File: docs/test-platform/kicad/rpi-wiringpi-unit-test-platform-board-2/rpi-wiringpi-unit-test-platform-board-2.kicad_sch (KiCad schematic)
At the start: 22 parts, among them J1 IN_PWR, J2 IN_SIGNAL, J3 IN_CS_SHIFTREG, J4 OUT_SERVO, J5 OUT_SERVO_SIG, SW1 SW_BOARD_CONN_LED, U1 MCP3008, U2 MCP4922, U3 MCP42010, U4 ADS1115, U5 74HC595

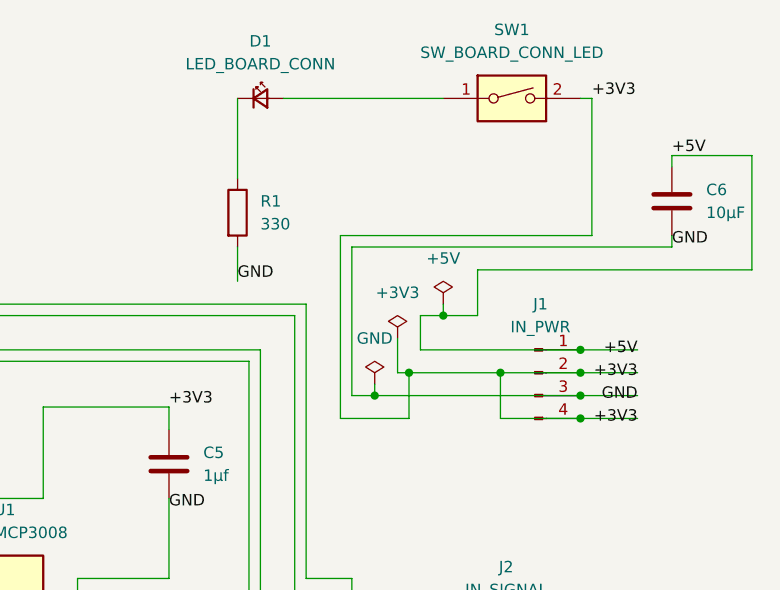
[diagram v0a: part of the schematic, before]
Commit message: Cleanup tracing
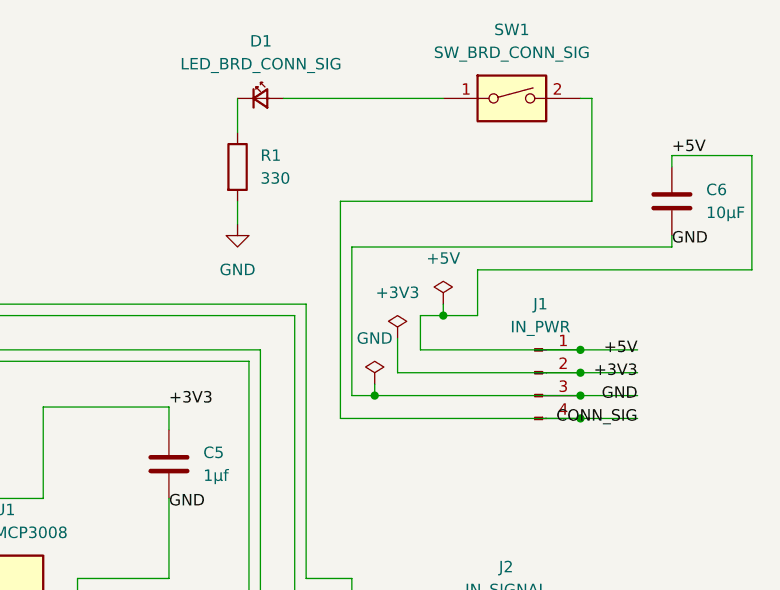
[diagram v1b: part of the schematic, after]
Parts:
- D1: value LED_BOARD_CONN -> LED_BRD_CONN_SIG
- SW1: value SW_BOARD_CONN_LED -> SW_BRD_CONN_SIG
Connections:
- net +3V3: no longer J1.4 (Pin_4), SW1.2
- new net CONN_SIG: J1.4 (Pin_4), SW1.2
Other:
- moved on the sheet: R1
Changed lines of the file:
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@@
 	)
 	(junction
-		(at 187.96 64.77)
-		(diameter 0)
-		(color 0 0 0 0)
-	)
-	(junction
 		(at 134.62 137.16)
 		(diameter 0)
@@
 	)
 	(junction
-		(at 207.01 69.85)
-		(diameter 0)
-		(color 0 0 0 0)
-	)
-	(junction
 		(at 207.01 67.31)
 		(diameter 0)
@@
 	)
 	(junction
+		(at 207.01 69.85)
+		(diameter 0)
+		(color 0 0 0 0)
+	)
+	(junction
 		(at 203.2 135.89)
 		(diameter 0)
@@
 	)
 	(junction
-		(at 198.12 64.77)
-		(diameter 0)
-		(color 0 0 0 0)
-	)
-	(junction
 		(at 203.2 128.27)
 		(diameter 0)
@@
 	(wire
 		(pts
-			(xy 208.28 34.29) (xy 208.28 49.53)
+			(xy 208.28 34.29) (xy 208.28 45.72)
 		)
 		(stroke
@@
 	(wire
 		(pts
-			(xy 208.28 49.53) (xy 180.34 49.53)
+			(xy 208.28 45.72) (xy 180.34 45.72)
 		)
 		(stroke
@@
 	(wire
 		(pts
-			(xy 168.91 34.29) (xy 168.91 43.18)
+			(xy 168.91 34.29) (xy 168.91 38.1)
 		)
 		(stroke
@@
 	(wire
 		(pts
-			(xy 187.96 64.77) (xy 198.12 64.77)
-		)
-		(stroke
-			(width 0)
-			(type default)
-		)
-	)
-	(wire
-		(pts
 			(xy 162.56 179.07) (xy 162.56 147.32)
 		)
@@
 	(wire
 		(pts
-			(xy 198.12 64.77) (xy 207.01 64.77)
-		)
-		(stroke
-			(width 0)
-			(type default)
-		)
-	)
-	(wire
-		(pts
 			(xy 170.18 63.5) (xy 170.18 92.71)
 		)
@@
 	(wire
 		(pts
-			(xy 198.12 69.85) (xy 207.01 69.85)
-		)
-		(stroke
-			(width 0)
-			(type default)
-		)
-	)
-	(wire
-		(pts
 			(xy 111.76 113.03) (xy 111.76 105.41)
 		)
@@
 	(wire
 		(pts
-			(xy 198.12 64.77) (xy 198.12 69.85)
-		)
-		(stroke
-			(width 0)
-			(type default)
-		)
-	)
-	(wire
-		(pts
 			(xy 161.29 78.74) (xy 161.29 87.63)
 		)
@@
 	(wire
 		(pts
+			(xy 168.91 45.72) (xy 168.91 48.26)
+		)
+		(stroke
+			(width 0)
+			(type default)
+		)
+	)
+	(wire
+		(pts
 			(xy 184.15 95.25) (xy 184.15 96.52)
 		)
@@
 	(wire
 		(pts
+			(xy 186.69 64.77) (xy 207.01 64.77)
+		)
+		(stroke
+			(width 0)
+			(type default)
+		)
+	)
+	(wire
+		(pts
 			(xy 22.86 77.47) (xy 22.86 87.63)
 		)
@@
 	(wire
 		(pts
-			(xy 180.34 69.85) (xy 187.96 69.85)
+			(xy 180.34 69.85) (xy 207.01 69.85)
 		)
 		(stroke
@@
 	(wire
 		(pts
-			(xy 186.69 64.77) (xy 187.96 64.77)
-		)
-		(stroke
-			(width 0)
-			(type default)
-		)
-	)
-	(wire
-		(pts
 			(xy 111.76 105.41) (xy 119.38 105.41)
 		)
@@
 	(wire
 		(pts
-			(xy 180.34 49.53) (xy 180.34 69.85)
+			(xy 180.34 45.72) (xy 180.34 69.85)
 		)
 		(stroke
@@
 	(wire
 		(pts
-			(xy 187.96 64.77) (xy 187.96 69.85)
-		)
-		(stroke
-			(width 0)
-			(type default)
-		)
-	)
-	(wire
-		(pts
 			(xy 208.28 152.4) (xy 208.28 146.05)
 		)
@@
 	(wire
 		(pts
-			(xy 168.91 50.8) (xy 168.91 54.61)
-		)
-		(stroke
-			(width 0)
-			(type default)
-		)
-	)
-	(wire
-		(pts
 			(xy 194.31 111.76) (xy 194.31 104.14)
 		)
@@
 		)
 	)
-	(label "+3V3"
+	(label "CONN_SIG"
 		(at 213.36 69.85 180)
 		(effects
@@
 		)
 	)
-	(label "+3V3"
-		(at 208.28 34.29 0)
-		(effects
-			(font
-				(size 1.27 1.27)
-			)
-			(justify left bottom)
-		)
-	)
 	(label "I2C_SDA"
 		(at 205.74 91.44 0)
@@
 		)
 	)
-	(label "GND"
-		(at 168.91 54.61 0)
-		(effects
-			(font
-				(size 1.27 1.27)
-			)
-			(justify left bottom)
-		)
-	)
 	(label "DAC_A_CH1"
 		(at 105.41 90.17 0)
@@
 	(symbol
 		(lib_id "Device:R")
-		(at 168.91 46.99 0)
+		(at 168.91 41.91 0)
 		(unit 1)
 		(body_style 1)
@@
 		(fields_autoplaced yes)
 		(property "Reference" "R1"
-			(at 171.45 45.72 0)
+			(at 171.45 40.64 0)
 			(show_name no)
 			(do_not_autoplace no)
@@
 		)
 		(property "Value" "330"
-			(at 171.45 48.26 0)
+			(at 171.45 43.18 0)
 			(show_name no)
 			(do_not_autoplace no)
@@
 		)
 		(property "Footprint" "Resistor_THT:R_Axial_DIN0207_L6.3mm_D2.5mm_P7.62mm_Horizontal"
-			(at 167.64 46.99 90)
+			(at 167.64 41.91 90)
 			(hide yes)
 			(show_name no)
@@
 		)
 		(property "Datasheet" ""
-			(at 168.91 46.99 0)
+			(at 168.91 41.91 0)
 			(hide yes)
 			(show_name no)
@@
 		)
 		(property "Description" "Resistor"
-			(at 168.91 46.99 0)
+			(at 168.91 41.91 0)
 			(hide yes)
 			(show_name no)
@@
 		)
 		(property "KiLib_Generator" "resistor/THT"
-			(at 168.91 46.99 0)
+			(at 168.91 41.91 0)
 			(hide yes)
 			(show_name no)
@@
 			)
 		)
-		(property "Value" "SW_BOARD_CONN_LED"
+		(property "Value" "SW_BRD_CONN_SIG"
 			(at 199.39 29.21 0)
 			(show_name no)
@@
 		(fields_autoplaced yes)
 		(property "Reference" "D1"
-			(at 171.45 27.94 0)
+			(at 171.5135 27.94 0)
 			(show_name no)
 			(do_not_autoplace no)
@@
 			)
 		)
-		(property "Value" "LED_BOARD_CONN"
-			(at 171.45 30.48 0)
+		(property "Value" "LED_BRD_CONN_SIG"
+			(at 171.5135 30.48 0)
 			(show_name no)
 			(do_not_autoplace no)
@@
 					(unit 1)
 				)
+			)
+		)
+	)
+	(symbol
+		(lib_id "power:GND")
+		(at 168.91 48.26 0)
+		(unit 1)
+		(body_style 1)
+		(exclude_from_sim no)
+		(in_bom yes)
+		(on_board yes)
+		(in_pos_files yes)
+		(dnp no)
+		(fields_autoplaced yes)
+		(property "Reference" "#PWR019"
+			(at 168.91 54.61 0)
+			(hide yes)
+			(show_name no)
+			(do_not_autoplace no)
+			(effects
+				(font
+					(size 1.27 1.27)
+				)
+			)
+		)
+		(property "Value" "GND"
+			(at 168.91 53.34 0)
+			(show_name no)
+			(do_not_autoplace no)
+			(effects
+				(font
+					(size 1.27 1.27)
+				)
+			)
+		)
+		(property "Footprint" ""
+			(at 168.91 48.26 0)
+			(hide yes)
+			(show_name no)
+			(do_not_autoplace no)
+			(effects
+				(font
+					(size 1.27 1.27)
+				)
+			)
+		)
+		(property "Datasheet" ""
+			(at 168.91 48.26 0)
+			(hide yes)
+			(show_name no)
+			(do_not_autoplace no)
+			(effects
+				(font
+					(size 1.27 1.27)
+				)
+			)
+		)
+		(property "Description" "Power symbol creates a global label with name \"GND\" , ground"
+			(at 168.91 48.26 0)
+			(hide yes)
+			(show_name no)
+			(do_not_autoplace no)
+			(effects
+				(font
+					(size 1.27 1.27)
+				)
+			)
+		)
+		(pin "1"
+		)
+		(instances
+			(project "rpi-wiringpi-unit-test-platform-board-2"
+				(path "/7946ceed-5e50-51f0-9396-19e4533fa9f5"
+					(reference "#PWR019")
+					(unit 1)
+				)
